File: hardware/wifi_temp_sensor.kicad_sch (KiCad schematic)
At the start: 12 parts, among them J1 USB_B_Mini, J2 ESP8266, J3 TempSensor, J4 Prog, J5 Aux_I2C, SW1 BootMode, U2 AZ1117-3.3

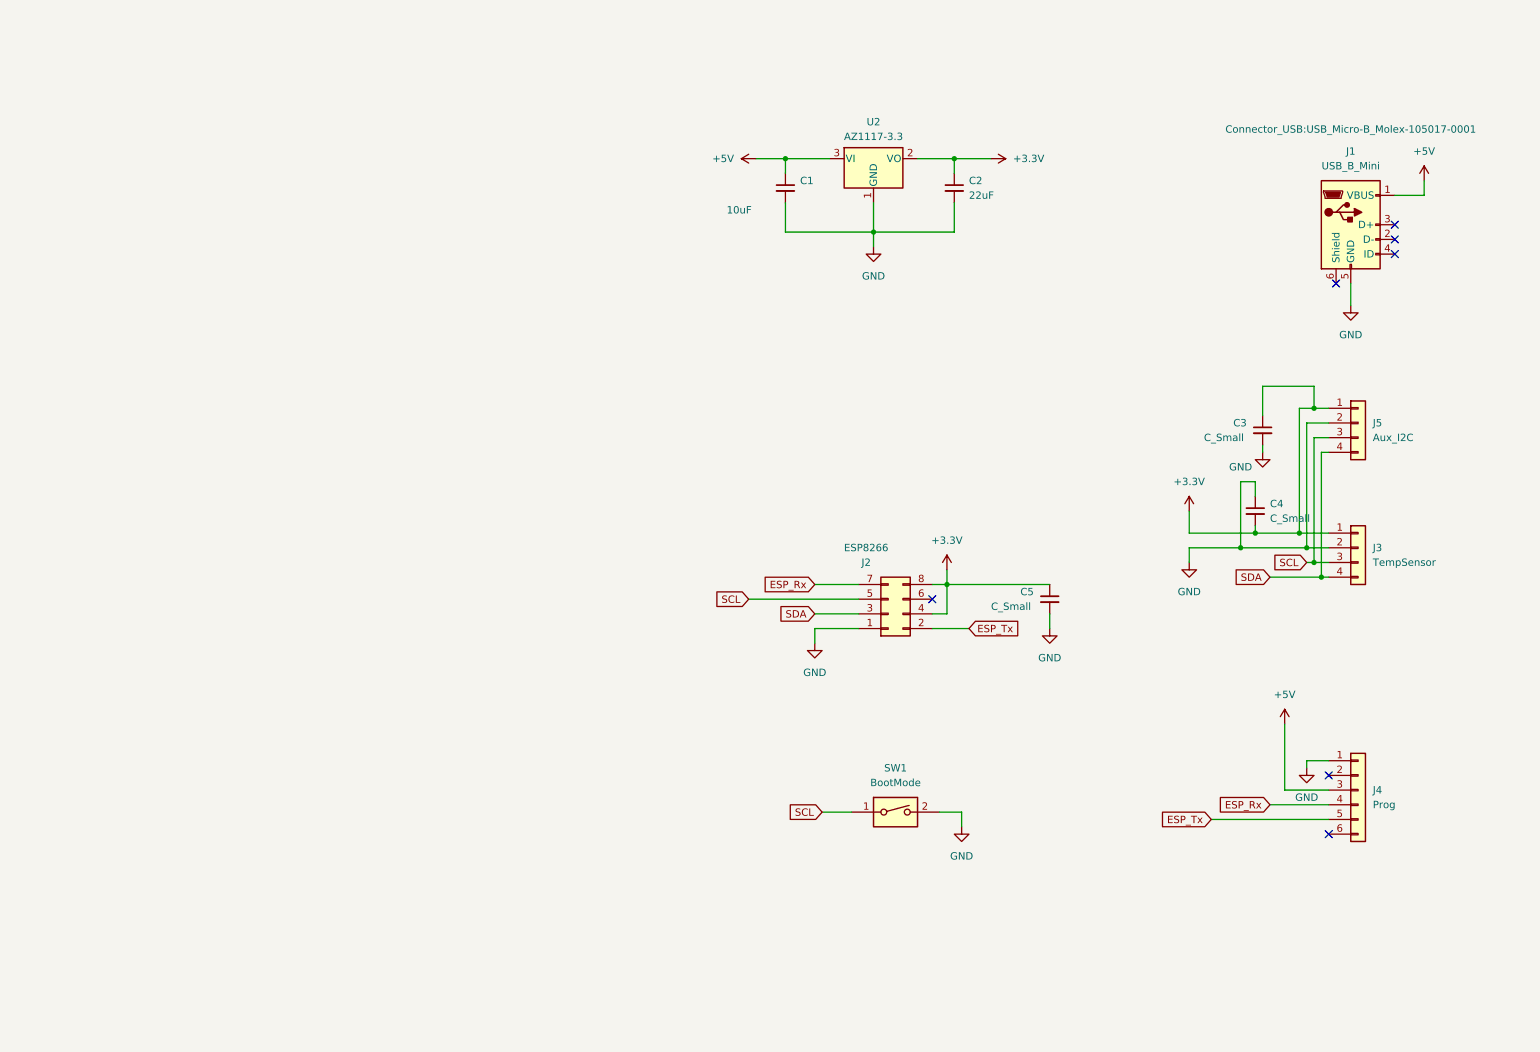
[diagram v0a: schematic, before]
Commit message: manual merge from esp32_msf_rcnotes
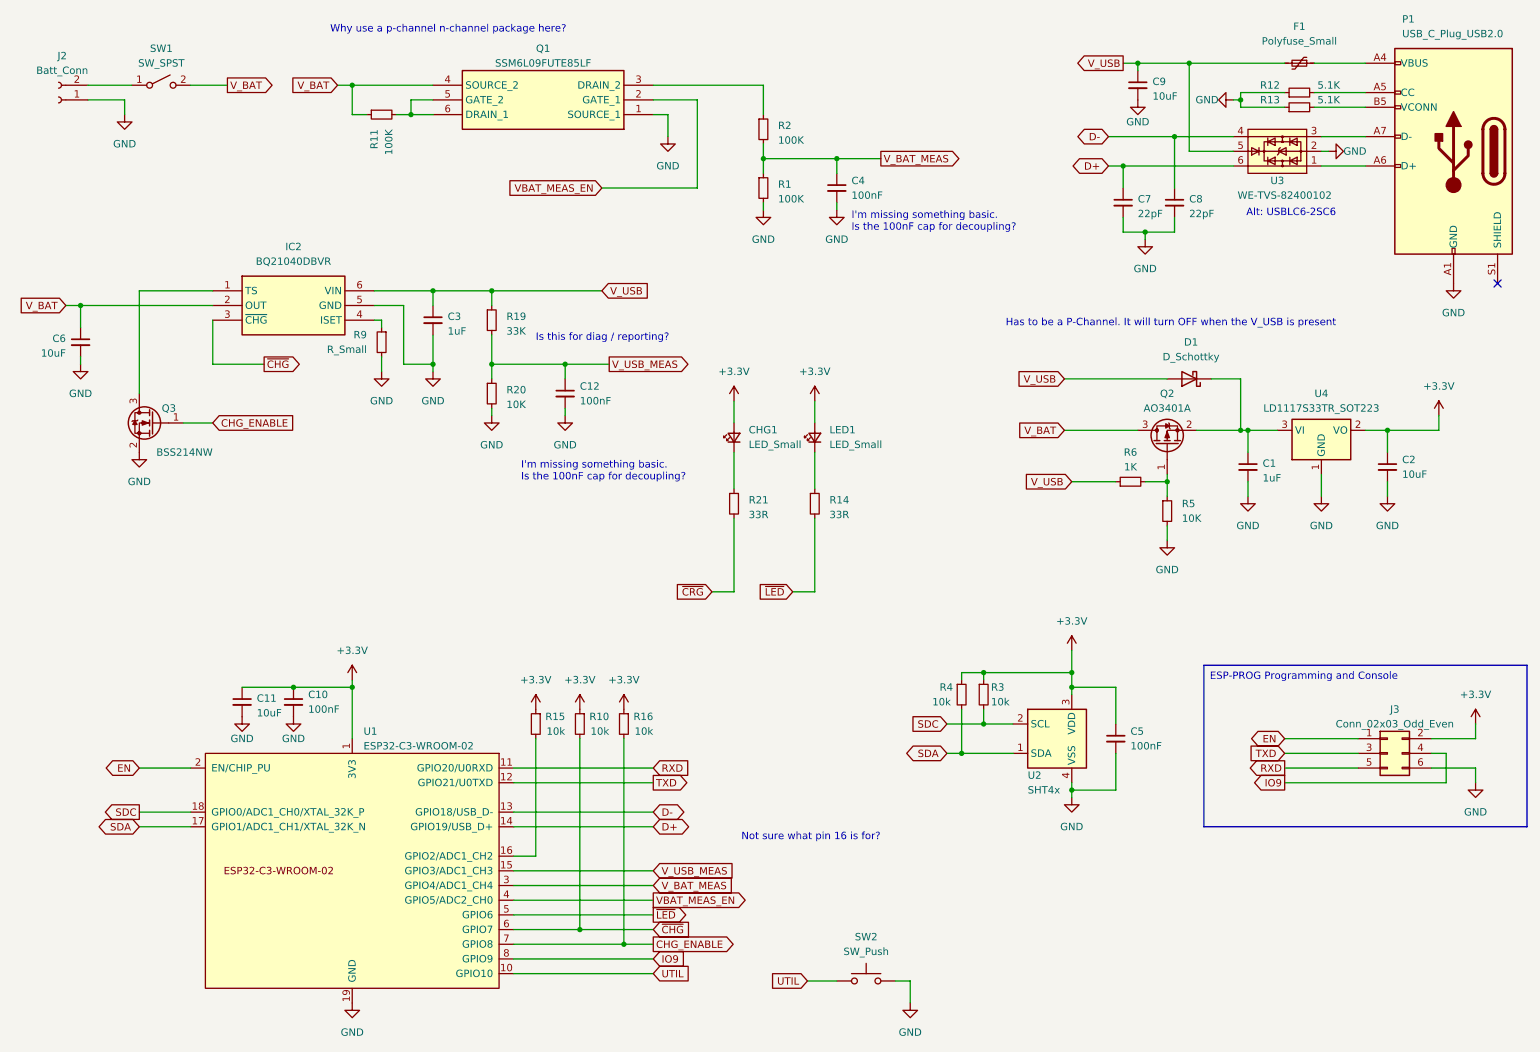
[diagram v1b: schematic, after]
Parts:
- removed J1: USB_B_Mini, Connector_USB:USB_Micro-B_Molex-105017-0001, symbol Connector:USB_B_Mini
- removed J2: ESP8266, Connector_PinSocket_2.54mm:PinSocket_2x04_P2.54mm_Vertical, symbol Connector_Generic:Conn_02x04_Odd_Even
- removed J3: TempSensor, Connector_PinSocket_2.54mm:PinSocket_1x04_P2.54mm_Vertical, symbol Connector_Generic:Conn_01x04
- removed J4: Prog, Connector_PinHeader_2.54mm:PinHeader_1x06_P2.54mm_Vertical, symbol Connector_Generic:Conn_01x06
- removed J5: Aux_I2C, Connector_PinSocket_2.54mm:PinSocket_1x04_P2.54mm_Vertical, symbol Connector_Generic:Conn_01x04
- removed SW1: BootMode, Button_Switch_THT:SW_PUSH_6mm, symbol Switch:SW_DIP_x01
- removed U2: AZ1117-3.3, Package_TO_SOT_SMD:SOT-89-3, symbol Regulator_Linear:AZ1117-3.3
- added C10, C12: 100nF, Capacitor_SMD:C_0603_1608Metric, symbol Device:C_Small
- added C11, C6, C9: 10uF, Capacitor_SMD:C_0805_2012Metric, symbol Device:C_Small
- added C7, C8: 22pF, Capacitor_SMD:C_0603_1608Metric, symbol Device:C_Small
- added CHG1, LED1: LED_Small, LED_SMD:LED_0603_1608Metric, symbol Device:LED_Small
- added D1: D_Schottky, Diode_SMD:D_0603_1608Metric, symbol Device:D_Schottky
- added F1: Polyfuse_Small, Fuse:Fuse_0603_1608Metric, symbol Device:Polyfuse_Small
- added IC2: BQ21040DBVR, SOT95P280X145-6N, symbol BQ21040DBVR:BQ21040DBVR
- added J2: Batt_Conn, Connector_JST:JST_ACH_BM02B-ACHSS-GAN-ETF_1x02-1MP_P1.20mm_Vertical, symbol Connector:Conn_01x02_Socket
- added J3: Conn_02x03_Odd_Even, Connector_PinHeader_1.27mm:PinHeader_2x03_P1.27mm_Vertical, symbol Connector_Generic:Conn_02x03_Odd_Even
- added P1: USB_C_Plug_USB2.0, Connector_USB:USB_C_Receptacle_Palconn_UTC16-G, symbol Connector:USB_C_Plug_USB2.0
- added Q1: SSM6L09FUTE85LF, SamacSys_parts:SOT65P210X120-6N, symbol SamacSys_parts:SSM6L09FUTE85LF
- added Q2: AO3401A, Package_TO_SOT_SMD:SOT-23, symbol Transistor_FET:AO3401A
- added Q3: BSS214NW, Package_TO_SOT_SMD:SOT-323_SC-70, symbol Transistor_FET:BSS214NW
- added R1, R2: 100K, Resistor_SMD:R_0603_1608Metric, symbol Device:R_Small
- added R10, R15, R16, R3, R4: 10k, Resistor_SMD:R_0603_1608Metric, symbol Device:R_Small
- added R11: 100K, Resistor_SMD:R_0402_1005Metric, symbol Device:R_Small
- added R12, R13: 5.1K, Resistor_SMD:R_0603_1608Metric, symbol Device:R_Small
- added R14, R21: 33R, Resistor_SMD:R_0603_1608Metric, symbol Device:R_Small
- added R19: 33K, Resistor_SMD:R_0603_1608Metric, symbol Device:R_Small
- added R20, R5: 10K, Resistor_SMD:R_0603_1608Metric, symbol Device:R_Small
- added R6: 1K, Resistor_SMD:R_0603_1608Metric, symbol Device:R_Small
- added R9: R_Small, Resistor_SMD:R_0603_1608Metric, symbol Device:R_Small
- added SW1: SW_SPST, Button_Switch_SMD:SW_SPDT_CK-JS102011SAQN, symbol Switch:SW_SPST
- added SW2: SW_Push, Button_Switch_SMD:SW_SPST_B3U-3000P, symbol Switch:SW_Push
- added U1: ESP32-C3-WROOM-02, PCM_Espressif:ESP32-C3-WROOM-02, symbol PCM_Espressif:ESP32-C3-WROOM-02
- added U2: SHT4x, Sensor_Humidity:Sensirion_DFN-4_1.5x1.5mm_P0.8mm_SHT4x_NoCentralPad, symbol Sensor_Humidity:SHT4x
- added U3: WE-TVS-82400102, Package_TO_SOT_SMD:SOT-23-6, symbol Power_Protection:WE-TVS-82400102
- added U4: LD1117S33TR_SOT223, Package_TO_SOT_SMD:SOT-223-3_TabPin2, symbol Regulator_Linear:LD1117S33TR_SOT223
- C1: value 10uF -> 1uF; footprint Capacitor_SMD:C_1206_3216Metric -> Capacitor_SMD:C_0603_1608Metric
- C2: value 22uF -> 10uF; footprint Capacitor_SMD:C_1206_3216Metric -> Capacitor_SMD:C_0805_2012Metric
- C3: value C_Small -> 1uF; footprint Capacitor_SMD:C_1206_3216Metric -> Capacitor_SMD:C_0603_1608Metric
- C4: value C_Small -> 100nF; footprint Capacitor_SMD:C_1206_3216Metric -> Capacitor_SMD:C_0603_1608Metric
- C5: value C_Small -> 100nF; footprint Capacitor_SMD:C_1206_3216Metric -> Capacitor_SMD:C_0402_1005Metric
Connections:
- net +3.3V: now also C10.1, C11.1, CHG1.2 (A), J3.2 (Pin_2), LED1.2 (A), R10.1, R15.1, R16.1, R3.1, R4.1, U1.1 (3V3), U2.3 (VDD), U4.2 (VO); no longer C3.1, C4.2
- net GND: now also C4.2, C10.2, C11.2, C12.2, C6.2, C7.2, C8.2, C9.2, IC2.5 (GND), J2.1 (Pin_1), J3.6 (Pin_6), P1.A1 (GND), P1.A12 (GND), P1.B1 (GND), P1.B12 (GND), Q1.1 (SOURCE_1), Q3.2 (S), R1.2, R12.1, R13.1, R20.2, R5.2, R9.2, SW2.2, U1.19 (GND), U1.9 (GND), U2.4 (VSS), U3.2, U4.1 (GND); no longer C4.1
- net SDA: now also R4.2, U1.17 (GPIO1/ADC1_CH1/XTAL_32K_N), U2.1 (SDA)
- net +5V: no longer names the net of C1.1
- net +5V: now also D1.1 (K), Q2.2 (S), U4.3 (VI)
- new net: P1.A6 (D+), U3.1
- new net: P1.A7 (D-), U3.3
- new net: F1.1, P1.A4 (VBUS), P1.A9 (VBUS), P1.B4 (VBUS), P1.B9 (VBUS)
- new net: R15.2, U1.16 (GPIO2/ADC1_CH2)
- new net: CHG1.1 (K), R21.1
- new net: Q2.1 (G), R5.1, R6.2
- new net: P1.B5 (VCONN), R13.2
- new net: Q1.3 (DRAIN_2), R2.1
- new net: Q1.5 (GATE_2), Q1.6 (DRAIN_1), R11.2
- new net: P1.A5 (CC), R12.2
- new net: IC2.4 (ISET), R9.1
- new net: IC2.1 (TS), Q3.3 (D)
- new net: J2.2 (Pin_2), SW1.1 (A)
- new net: LED1.1 (K), R14.1
- new net CHG_ENABLE: Q3.1 (G), R16.2, U1.7 (GPIO8)
- new net D+: C7.1, U1.14 (GPIO19/USB_D+), U3.6
- new net D-: C8.1, U1.13 (GPIO18/USB_D-), U3.4
- new net EN: J3.1 (Pin_1), U1.2 (EN/CHIP_PU)
- new net IO9: J3.4 (Pin_4), U1.8 (GPIO9)
- new net RXD: J3.5 (Pin_5), U1.11 (GPIO20/U0RXD)
- new net SDC: R3.2, U1.18 (GPIO0/ADC1_CH0/XTAL_32K_P), U2.2 (SCL)
- new net TXD: J3.3 (Pin_3), U1.12 (GPIO21/U0TXD)
- new net UTIL: SW2.1, U1.10 (GPIO10)
- new net VBAT_MEAS_EN: Q1.2 (GATE_1), U1.4 (GPIO5/ADC2_CH0)
- new net V_BAT: C6.1, IC2.2 (OUT), Q1.4 (SOURCE_2), Q2.3 (D), R11.1, SW1.2 (B)
- new net V_BAT_MEAS: C4.1, R1.1, R2.2, U1.3 (GPIO4/ADC1_CH4)
- new net V_USB: C3.1, C9.1, D1.2 (A), F1.2, IC2.6 (VIN), R19.1, R6.1, U3.5
- new net V_USB_MEAS: C12.1, R19.2, R20.1, U1.15 (GPIO3/ADC1_CH3)
- new net ~{CHG}: IC2.3 (~{CHG}), R10.2, U1.6 (GPIO7)
- new net ~{CRG}: R21.2
- new net ~{LED}: R14.2, U1.5 (GPIO6)
- no-connect marks 7 -> 1
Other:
- note added: "Alt: USBLC6-2SC6"
- note added: "Has to be a P-Channel. It will turn OFF when the V_USB is present"
- note added: "I'm missing something basic. Is the 100nF cap for decoupling?"
- note added: "Is this for diag / reporting?"
- note added: "Not sure what pin 16 is for?"
- note added: "Why use a p-channel n-channel package here?"
